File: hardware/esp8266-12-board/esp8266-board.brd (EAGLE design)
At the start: 24.9 x 40 mm, 16 parts, among them P1 ESP8266, P2 ESP8266 CONNECTOR, T1 AMS1117, T2 LM7805

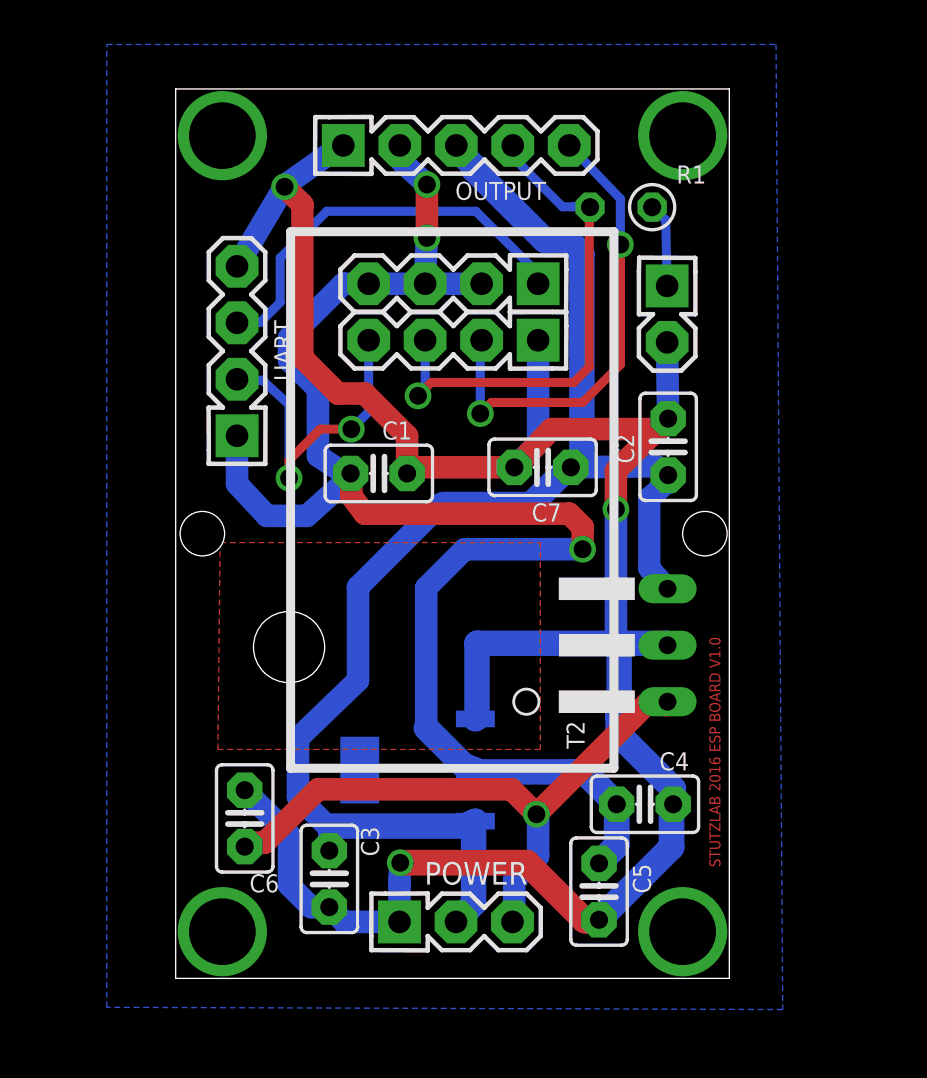
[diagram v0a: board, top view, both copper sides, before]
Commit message: generic switch board creation
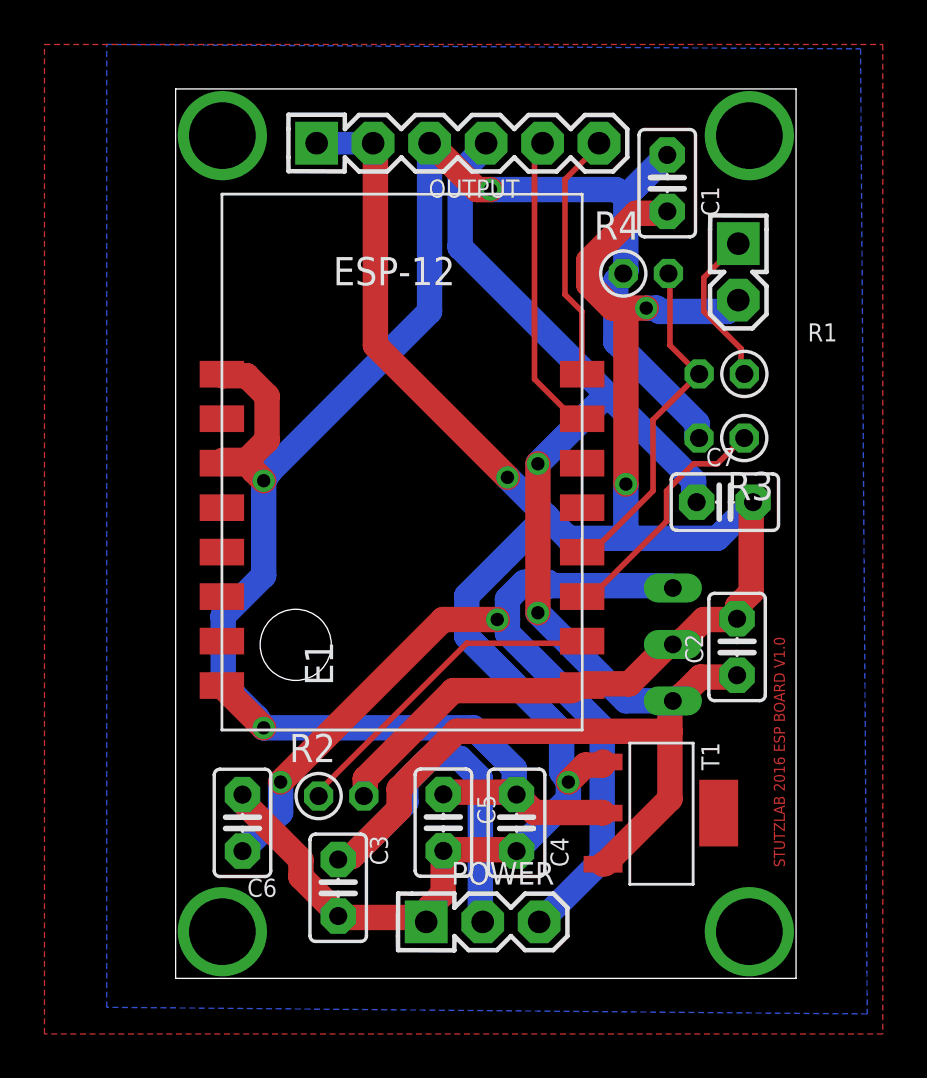
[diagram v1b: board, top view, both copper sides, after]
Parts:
- removed P1: ESP8266, stutz-eagle:PIN-HEADER-4PIN
- removed P2: ESP8266 CONNECTOR, stutz-eagle:PIN-HEADER-4PIN
- removed UART: 3.3V RX TX GND, stutz-eagle:PIN-HEADER-4PIN
- added E1: ESP8266-12, stutz-eagle:ESP8266-12
- added R2, R3: 3k3, stutz-eagle:RESISTOR-V1
- added R4: 10k, stutz-eagle:RESISTOR-V1
- OUTPUT: value GND 3.3V 5V IO0 IO2 -> GND GND 3.3V 5V RX TX; device stutz-eagle:PIN-HEADER-5PIN -> stutz-eagle:PIN-HEADER-6PIN
- R1: value 3k3 -> 470; device stutz-eagle:RESISTOR-V2 -> stutz-eagle:RESISTOR-V1
- moved C1 18.4 mm to (22.1, 35.8), turned to 270 degrees
- moved T1 11.1 mm to (21.8, 7.43), flipped to the top
- moved C2 9.52 mm to (25.2, 14.9)
- moved R1 8.70 mm to (24.3, 27.2)
- moved C7 8.35 mm to (24.7, 21.4), turned to 0 degrees
- moved C5 7.66 mm to (12.0, 7.01)
- moved C4 5.83 mm to (15.3, 7.00), turned to 270 degrees
- moved FIRMWARE 3.72 mm to (25.3, 31.8)
- moved OUTPUT 1.20 mm to (11.4, 37.6)
- moved POWER 1.20 mm to (13.8, 2.54)
- moved C3 0.57 mm to (7.31, 4.08)
- moved T2 0.24 mm to (13.5, 15.0), flipped to the bottom, turned to 270 degrees
- moved C6 0.22 mm to (3.01, 6.99)
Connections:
- new net ESP_GPIO15: E1.2, R2.1
- new net GPIO5: E1.6
- net +3.3V: now also E1.11, E1.16, E1.9, OUTPUT.3, R3.2, R4.1; no longer OUTPUT.2, P1.2, P1.3, P1.4, UART.1
- net +5V: now also OUTPUT.4; no longer OUTPUT.3
- net ESP_GPIO0: now also E1.4, R4.2; no longer OUTPUT.4, P2.3
- net ESP_GPIO2: now also E1.3, R3.1; no longer OUTPUT.5, P2.2
- net ESP_RX: now also E1.7, OUTPUT.5; no longer P2.4, UART.2
- net ESP_TX: now also E1.8, OUTPUT.6; no longer P1.1, UART.3
- net GND: now also E1.1, OUTPUT.2, R2.2; no longer P2.1, UART.4
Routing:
- net +5V: track 64.9 -> 85.5 mm, vias 0 -> 2
- net ESP_GPIO15: track 0.00 -> 15.0 mm
- net +24V: track 28.0 -> 42.4 mm, vias 1 -> 2
- net +3.3V: track 73.6 -> 87.5 mm
- net GND: track 108.1 -> 121.7 mm, vias 3 -> 4
- net ESP_GPIO2: track 21.3 -> 11.0 mm, vias 2 -> 0
- net ESP_GPIO0: track 22.9 -> 15.6 mm, vias 1 -> 0
- net ESP_TX: track 18.4 -> 11.3 mm
- net N$1: track 3.80 -> 7.30 mm
- net ESP_RX: track 14.6 -> 13.7 mm, vias 2 -> 0
- added copper zone on layer 1, net GND
- removed copper zone on layer 1, net N$6
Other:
- board size 24.9 x 40 mm -> 27.9 x 40 mm
